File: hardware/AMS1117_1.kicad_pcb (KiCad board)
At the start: 2 copper layers, 9 parts, among them J12 Conn_01x03, U4 AMS1117-3.3

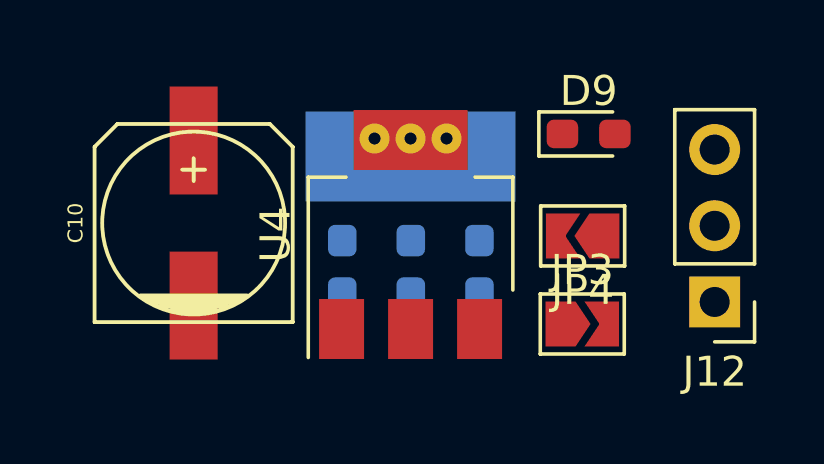
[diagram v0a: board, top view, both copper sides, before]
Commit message: update,
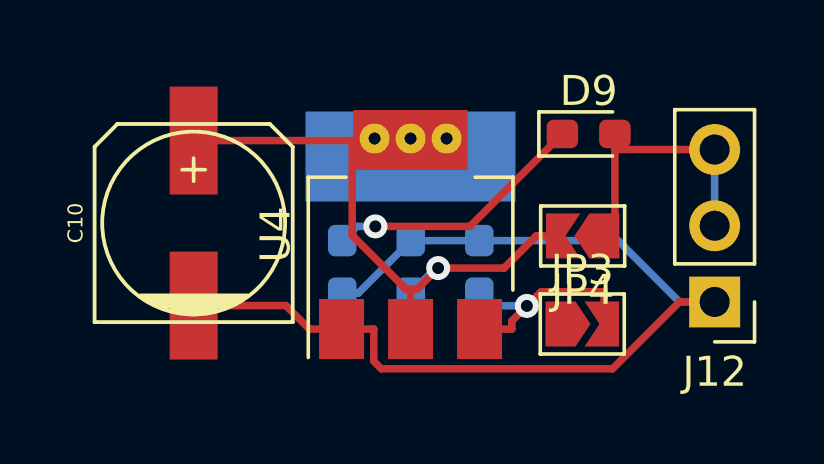
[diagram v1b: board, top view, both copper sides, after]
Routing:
- net GND: track 0.00 -> 33.8 mm
- net Net-(C10-Pad1): track 0.00 -> 22.7 mm, vias 0 -> 1
- net +3V3: track 0.00 -> 9.41 mm
- net Net-(D9-Pad1): track 0.00 -> 8.81 mm, vias 0 -> 1
- net Net-(C8-Pad1): track 0.00 -> 7.65 mm, vias 0 -> 1
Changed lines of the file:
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@@
     (thickness 1.6)
     (drawings 0)
-    (tracks 0)
+    (tracks 53)
     (zones 0)
     (modules 9)
@@
     (uvia_drill 0.1)
     (add_net +3V3)
-    (add_net +5V)
     (add_net GND)
     (add_net "Net-(C10-Pad1)")
@@
     )
   )
+  (segment (start 40.3 41.95) (end 39.2247 41.95) (width 0.25) (layer F.Cu) (net 1))
+  (segment (start 35.3695 41.1683) (end 38.443 41.1683) (width 0.25) (layer F.Cu) (net 1))
+  (segment (start 38.443 41.1683) (end 39.2247 41.95) (width 0.25) (layer F.Cu) (net 1))
+  (segment (start 40.3 41.95) (end 41.3753 41.95) (width 0.25) (layer F.Cu) (net 1))
+  (segment (start 52.7365 41.048) (end 51.5612 41.048) (width 0.25) (layer F.Cu) (net 1))
+  (segment (start 51.5612 41.048) (end 49.3338 43.2754) (width 0.25) (layer F.Cu) (net 1))
+  (segment (start 49.3338 43.2754) (end 41.6254 43.2754) (width 0.25) (layer F.Cu) (net 1))
+  (segment (start 41.6254 43.2754) (end 41.3753 43.0253) (width 0.25) (layer F.Cu) (net 1))
+  (segment (start 41.3753 43.0253) (end 41.3753 41.95) (width 0.25) (layer F.Cu) (net 1))
+  (segment (start 42.6085 39.003) (end 40.8585 40.753) (width 0.25) (layer B.Cu) (net 1))
+  (segment (start 40.8585 40.753) (end 40.3225 40.753) (width 0.25) (layer B.Cu) (net 1))
+  (segment (start 44.8945 39.003) (end 42.6085 39.003) (width 0.25) (layer B.Cu) (net 1))
+  (segment (start 51.5612 41.048) (end 49.5162 39.003) (width 0.25) (layer B.Cu) (net 1))
+  (segment (start 49.5162 39.003) (end 44.8945 39.003) (width 0.25) (layer B.Cu) (net 1))
+  (segment (start 52.7365 41.048) (end 51.5612 41.048) (width 0.25) (layer B.Cu) (net 1))
+  (segment (start 49.0485 40.7077) (end 46.9488 40.7077) (width 0.25) (layer F.Cu) (net 2))
+  (segment (start 46.9488 40.7077) (end 46.4764 41.1801) (width 0.25) (layer F.Cu) (net 2))
+  (segment (start 45.9753 41.95) (end 45.9753 41.6812) (width 0.25) (layer F.Cu) (net 2))
+  (segment (start 45.9753 41.6812) (end 46.4764 41.1801) (width 0.25) (layer F.Cu) (net 2))
+  (segment (start 44.8945 40.753) (end 45.3216 41.1801) (width 0.25) (layer B.Cu) (net 2))
+  (segment (start 45.3216 41.1801) (end 46.4764 41.1801) (width 0.25) (layer B.Cu) (net 2))
+  (segment (start 44.9 41.95) (end 45.9753 41.95) (width 0.25) (layer F.Cu) (net 2))
+  (segment (start 49.0485 41.783) (end 49.0485 40.7077) (width 0.25) (layer F.Cu) (net 2))
+  (via (at 46.4764 41.1801) (size 0.8) (layers F.Cu B.Cu) (net 2))
+  (segment (start 46.7862 38.848) (end 45.715 39.9192) (width 0.25) (layer F.Cu) (net 3))
+  (segment (start 45.715 39.9192) (end 43.5196 39.9192) (width 0.25) (layer F.Cu) (net 3))
+  (segment (start 43.5196 39.9192) (end 42.8141 40.6247) (width 0.25) (layer F.Cu) (net 3))
+  (segment (start 42.8141 40.6247) (end 42.6 40.6247) (width 0.25) (layer F.Cu) (net 3))
+  (segment (start 43.5196 39.9192) (end 43.4423 39.9192) (width 0.25) (layer B.Cu) (net 3))
+  (segment (start 43.4423 39.9192) (end 42.6085 40.753) (width 0.25) (layer B.Cu) (net 3))
+  (segment (start 40.6535 35.6667) (end 41.3333 35.6667) (width 0.25) (layer F.Cu) (net 3))
+  (segment (start 41.3333 35.6667) (end 41.4 35.6) (width 0.25) (layer F.Cu) (net 3))
+  (segment (start 35.3695 35.6667) (end 40.6535 35.6667) (width 0.25) (layer F.Cu) (net 3))
+  (segment (start 40.6535 35.6667) (end 40.6535 38.823) (width 0.25) (layer F.Cu) (net 3))
+  (segment (start 40.6535 38.823) (end 42.4552 40.6247) (width 0.25) (layer F.Cu) (net 3))
+  (segment (start 42.4552 40.6247) (end 42.6 40.6247) (width 0.25) (layer F.Cu) (net 3))
+  (segment (start 42.6 41.95) (end 42.6 40.6247) (width 0.25) (layer F.Cu) (net 3))
+  (segment (start 47.6115 38.848) (end 46.7862 38.848) (width 0.25) (layer F.Cu) (net 3))
+  (segment (start 42.6 35.6) (end 43.8 35.6) (width 0.25) (layer F.Cu) (net 3))
+  (segment (start 41.4 35.6) (end 42.6 35.6) (width 0.25) (layer F.Cu) (net 3))
+  (segment (start 42.6 35.65) (end 42.6 35.6) (width 0.25) (layer F.Cu) (net 3))
+  (via (at 43.5196 39.9192) (size 0.8) (layers F.Cu B.Cu) (net 3))
+  (segment (start 49.4115 35.968) (end 49.4115 38.498) (width 0.25) (layer F.Cu) (net 4))
+  (segment (start 49.4115 38.498) (end 49.0615 38.848) (width 0.25) (layer F.Cu) (net 4))
+  (segment (start 49.4115 35.448) (end 49.4115 35.968) (width 0.25) (layer F.Cu) (net 4))
+  (segment (start 49.4115 35.968) (end 51.5612 35.968) (width 0.25) (layer F.Cu) (net 4))
+  (segment (start 52.7365 35.968) (end 51.5612 35.968) (width 0.25) (layer F.Cu) (net 4))
+  (segment (start 52.7365 38.508) (end 52.7365 35.968) (width 0.25) (layer B.Cu) (net 4))
+  (segment (start 47.6615 35.448) (end 44.5795 38.53) (width 0.25) (layer F.Cu) (net 5))
+  (segment (start 44.5795 38.53) (end 41.4259 38.53) (width 0.25) (layer F.Cu) (net 5))
+  (segment (start 41.4259 38.53) (end 40.7955 38.53) (width 0.25) (layer B.Cu) (net 5))
+  (segment (start 40.7955 38.53) (end 40.3225 39.003) (width 0.25) (layer B.Cu) (net 5))
+  (via (at 41.4259 38.53) (size 0.8) (layers F.Cu B.Cu) (net 5))
 )
